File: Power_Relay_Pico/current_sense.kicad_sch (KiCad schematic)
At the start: 3 parts, among them J501 Conn_01x08_Pin, J502 Conn_01x08_Pin, U501 INA3221

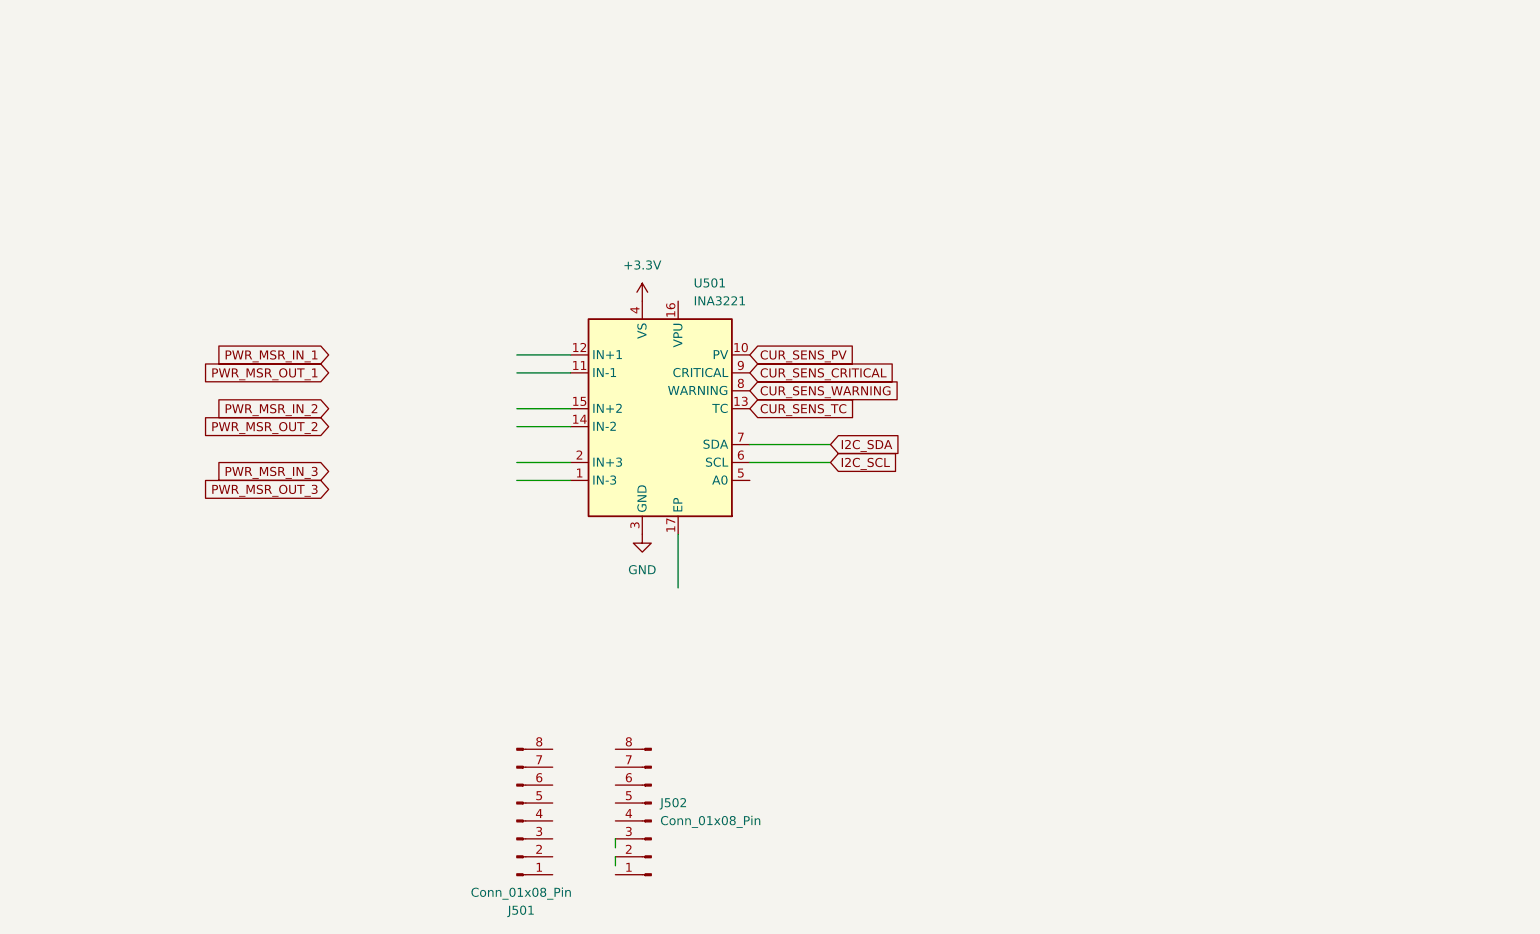
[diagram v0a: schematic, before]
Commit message: started routing
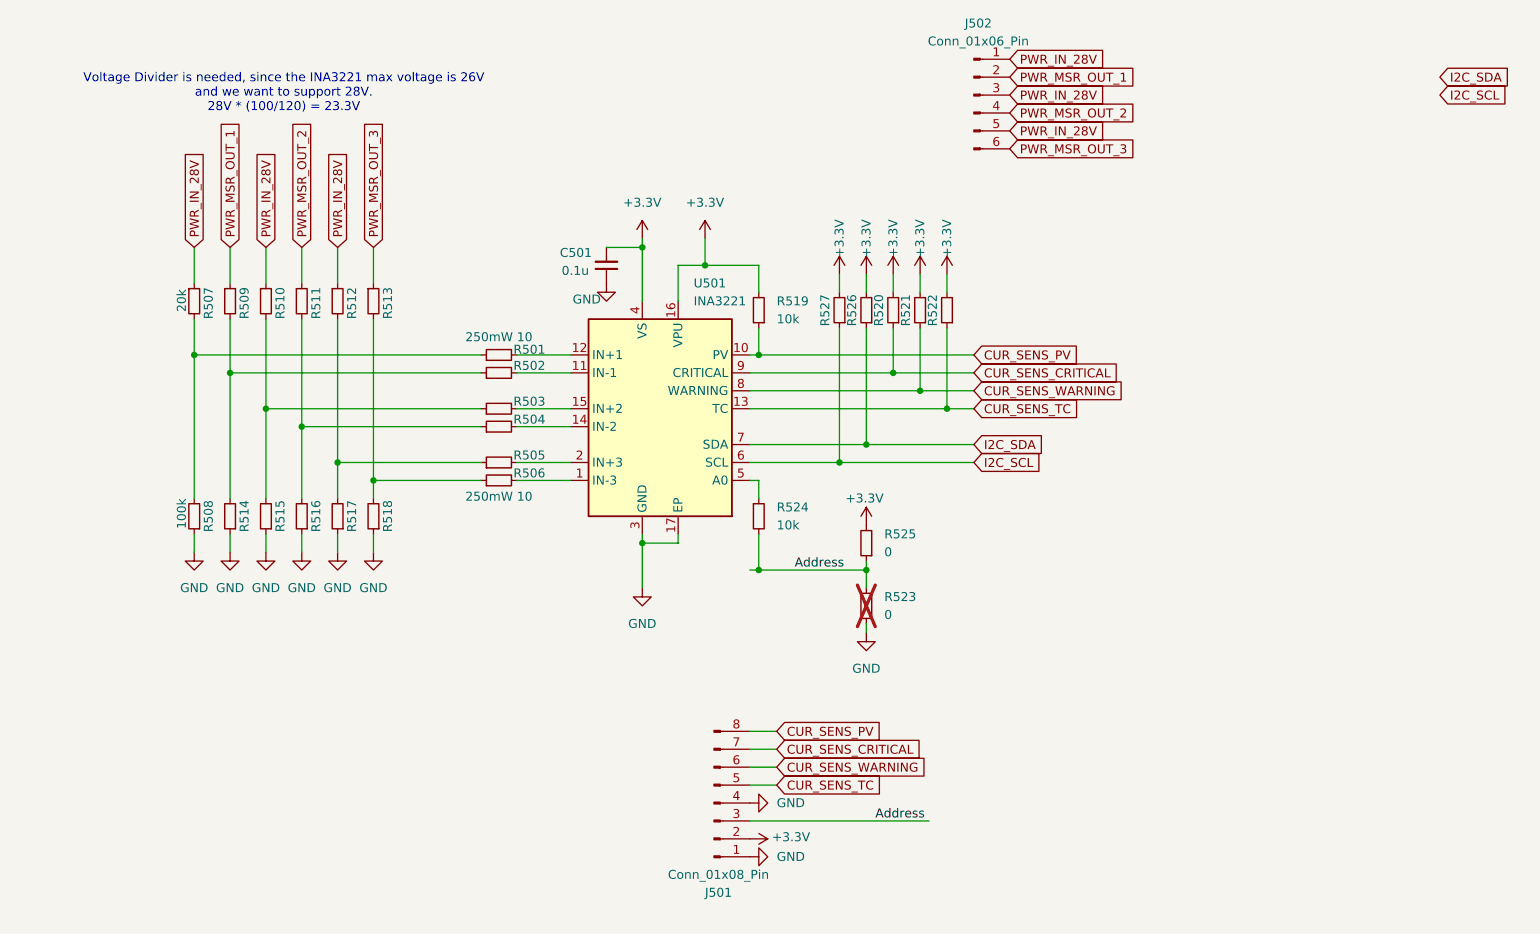
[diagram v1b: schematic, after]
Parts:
- removed J502: Conn_01x08_Pin, Connector_PinHeader_1.00mm:PinHeader_1x08_P1.00mm_Vertical, symbol Connector:Conn_01x08_Pin
- added C501: 0.1u, Capacitor_SMD:C_0603_1608Metric, symbol Device:C_Small
- added J502: Conn_01x06_Pin, Connector_PinHeader_1.00mm:PinHeader_1x06_P1.00mm_Vertical, symbol Connector:Conn_01x06_Pin
- added R501, R502, R503, R504, R505, R506: 250mW 10, Resistor_SMD:R_1206_3216Metric, symbol Device:R_Small
- added R507, R509, R510, R511, R512, R513: 20k, Resistor_SMD:R_0603_1608Metric, symbol Device:R_Small
- added R508, R514, R515, R516, R517, R518: 100k, Resistor_SMD:R_0603_1608Metric, symbol Device:R_Small
- added R519, R520, R521, R522, R524, R526, R527: 10k, Resistor_SMD:R_0603_1608Metric, symbol Device:R_Small
- added R523, R525: 0, Resistor_SMD:R_0603_1608Metric, symbol Device:R_Small
- J501: footprint Connector_PinHeader_1.00mm:PinHeader_1x08_P1.00mm_Vertical -> Connector_PinHeader_2.54mm:PinHeader_1x08_P2.54mm_Vertical; LCSC (none) -> --
- U501: LCSC (none) -> C181255
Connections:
- net +3.3V: now also J501.2 (Pin_2), U501.16 (VPU), C501.2, R519.2, R520.2, R521.2, R522.2, R525.2, R526.2, R527.2
- net CUR_SENS_CRITICAL: now also J501.7 (Pin_7), R520.1
- net CUR_SENS_PV: now also J501.8 (Pin_8), R519.1
- net CUR_SENS_TC: now also J501.5 (Pin_5), R522.1
- net CUR_SENS_WARNING: now also J501.6 (Pin_6), R521.1
- net GND: now also J501.1 (Pin_1), J501.4 (Pin_4), U501.17 (EP), C501.1, R508.1, R514.1, R515.1, R516.1, R517.1, R518.1, R523.1
- net I2C_SCL: now also R527.1
- net I2C_SDA: now also R526.1
- net PWR_MSR_OUT_1: now also J502.2 (Pin_2), R509.1
- net PWR_MSR_OUT_2: now also J502.4 (Pin_4), R511.1
- net PWR_MSR_OUT_3: now also J502.6 (Pin_6), R513.1
- net Address: now reaches J501.3 (Pin_3)
- net Address: now also R523.2, R524.2, R525.1
- net at U501.1 (IN-3): now also R506.2
- net at U501.11 (IN-1): now also R502.2
- net at U501.12 (IN+1): now also R501.2
- net at U501.14 (IN-2): now also R504.2
- net at U501.15 (IN+2): now also R503.2
- net at U501.2 (IN+3): now also R505.2
- net at U501.5 (A0): now also R524.1
- new net: R504.1, R511.2, R516.2
- new net: R506.1, R513.2, R518.2
- new net: R505.1, R512.2, R517.2
- new net: R502.1, R509.2, R514.2
- new net: R501.1, R507.2, R508.2
- new net: R503.1, R510.2, R515.2
- new net PWR_IN_28V: J502.1 (Pin_1), J502.3 (Pin_3), J502.5 (Pin_5), R507.1, R510.1, R512.1
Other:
- note added: "Voltage Divider is needed, since the INA3221 max voltage is 26V and we want to support 28V. 28V * (100/120) = 23.3V"
- moved on the sheet: J501

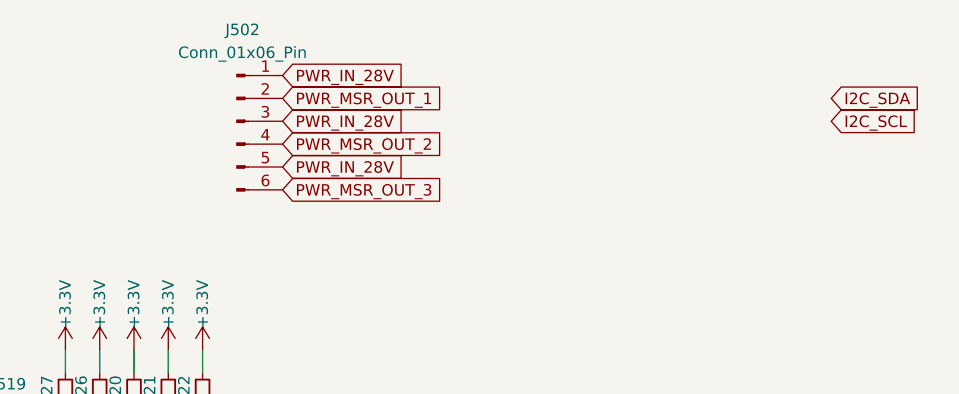
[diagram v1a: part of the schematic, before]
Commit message: as ordered
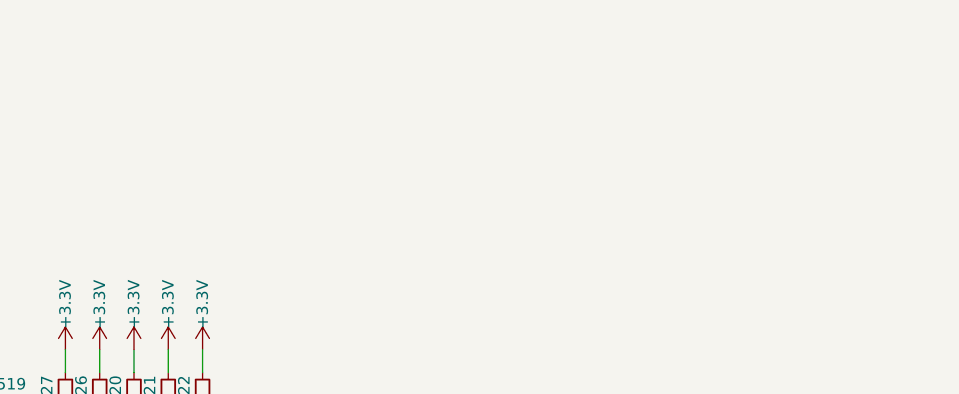
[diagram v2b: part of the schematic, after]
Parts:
- removed J502: Conn_01x06_Pin, Connector_PinHeader_1.00mm:PinHeader_1x06_P1.00mm_Vertical, symbol Connector:Conn_01x06_Pin
